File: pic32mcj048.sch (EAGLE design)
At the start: 14 parts

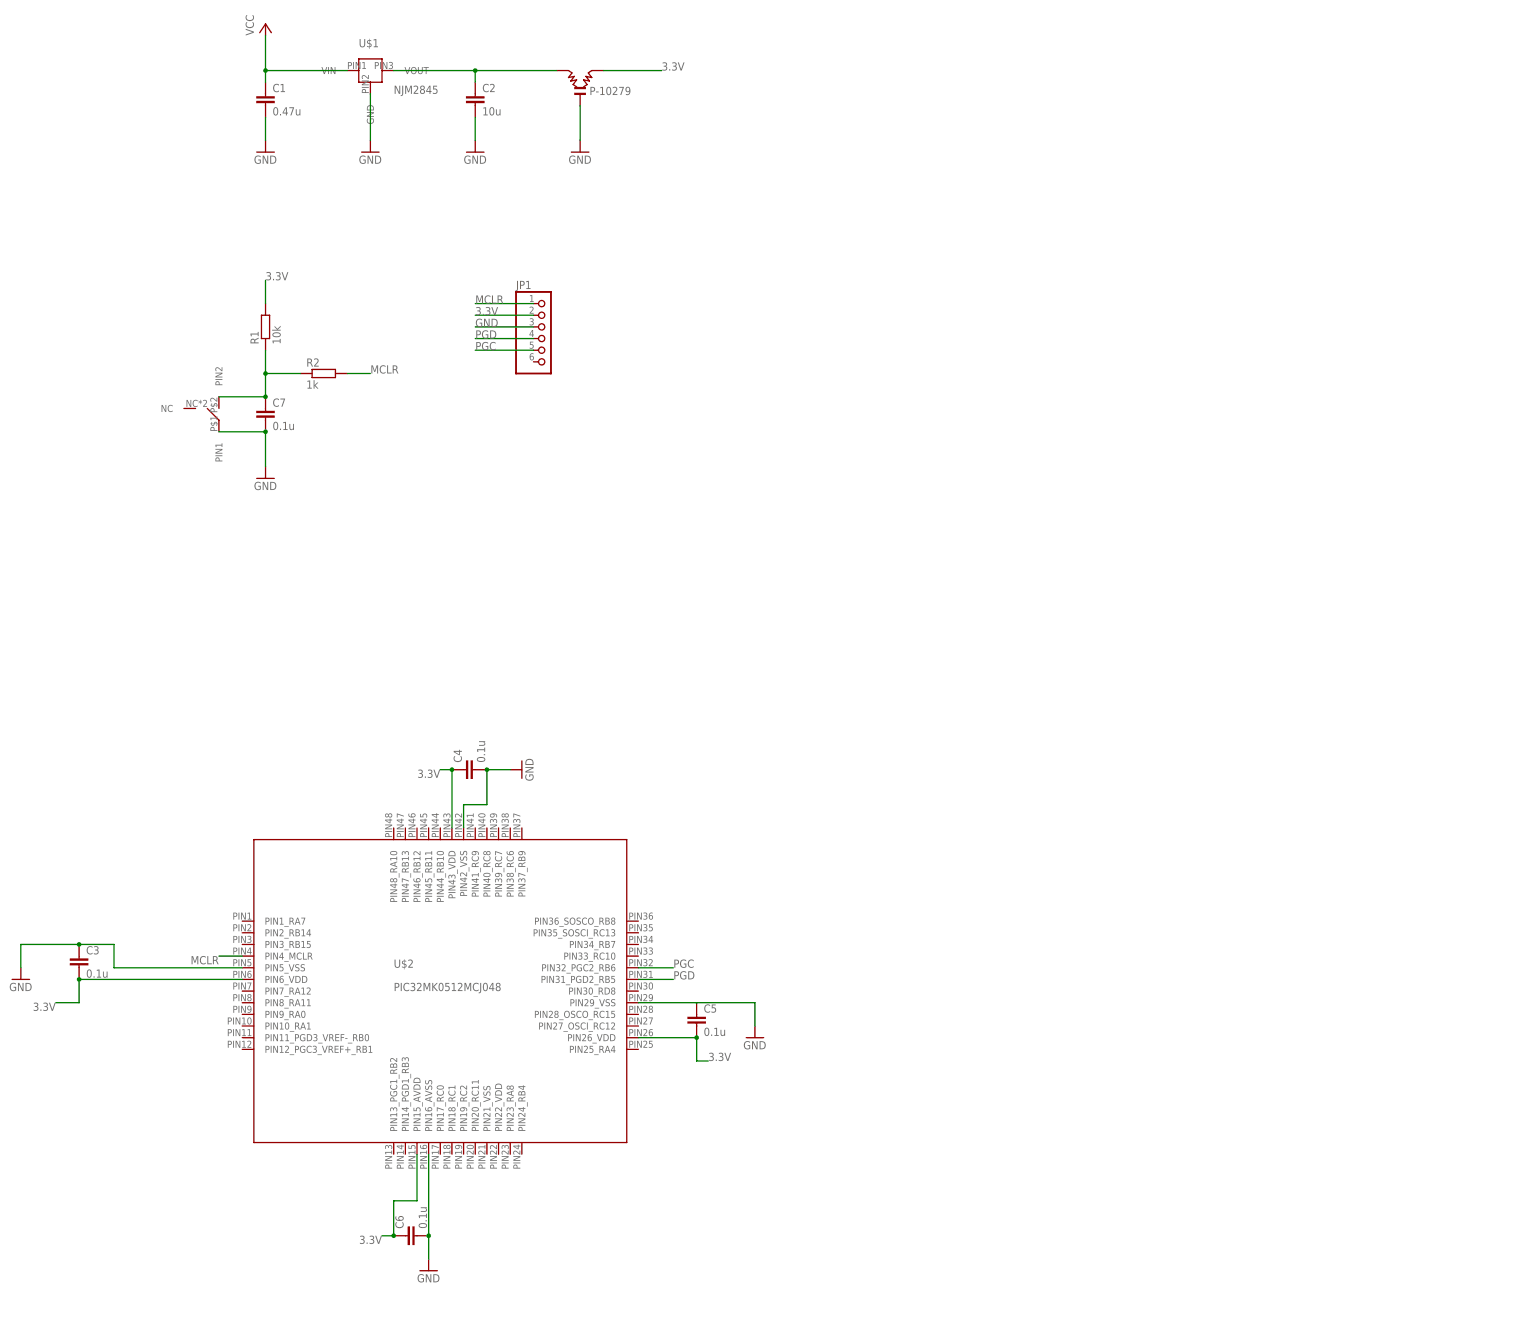
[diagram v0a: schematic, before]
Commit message: sch完成
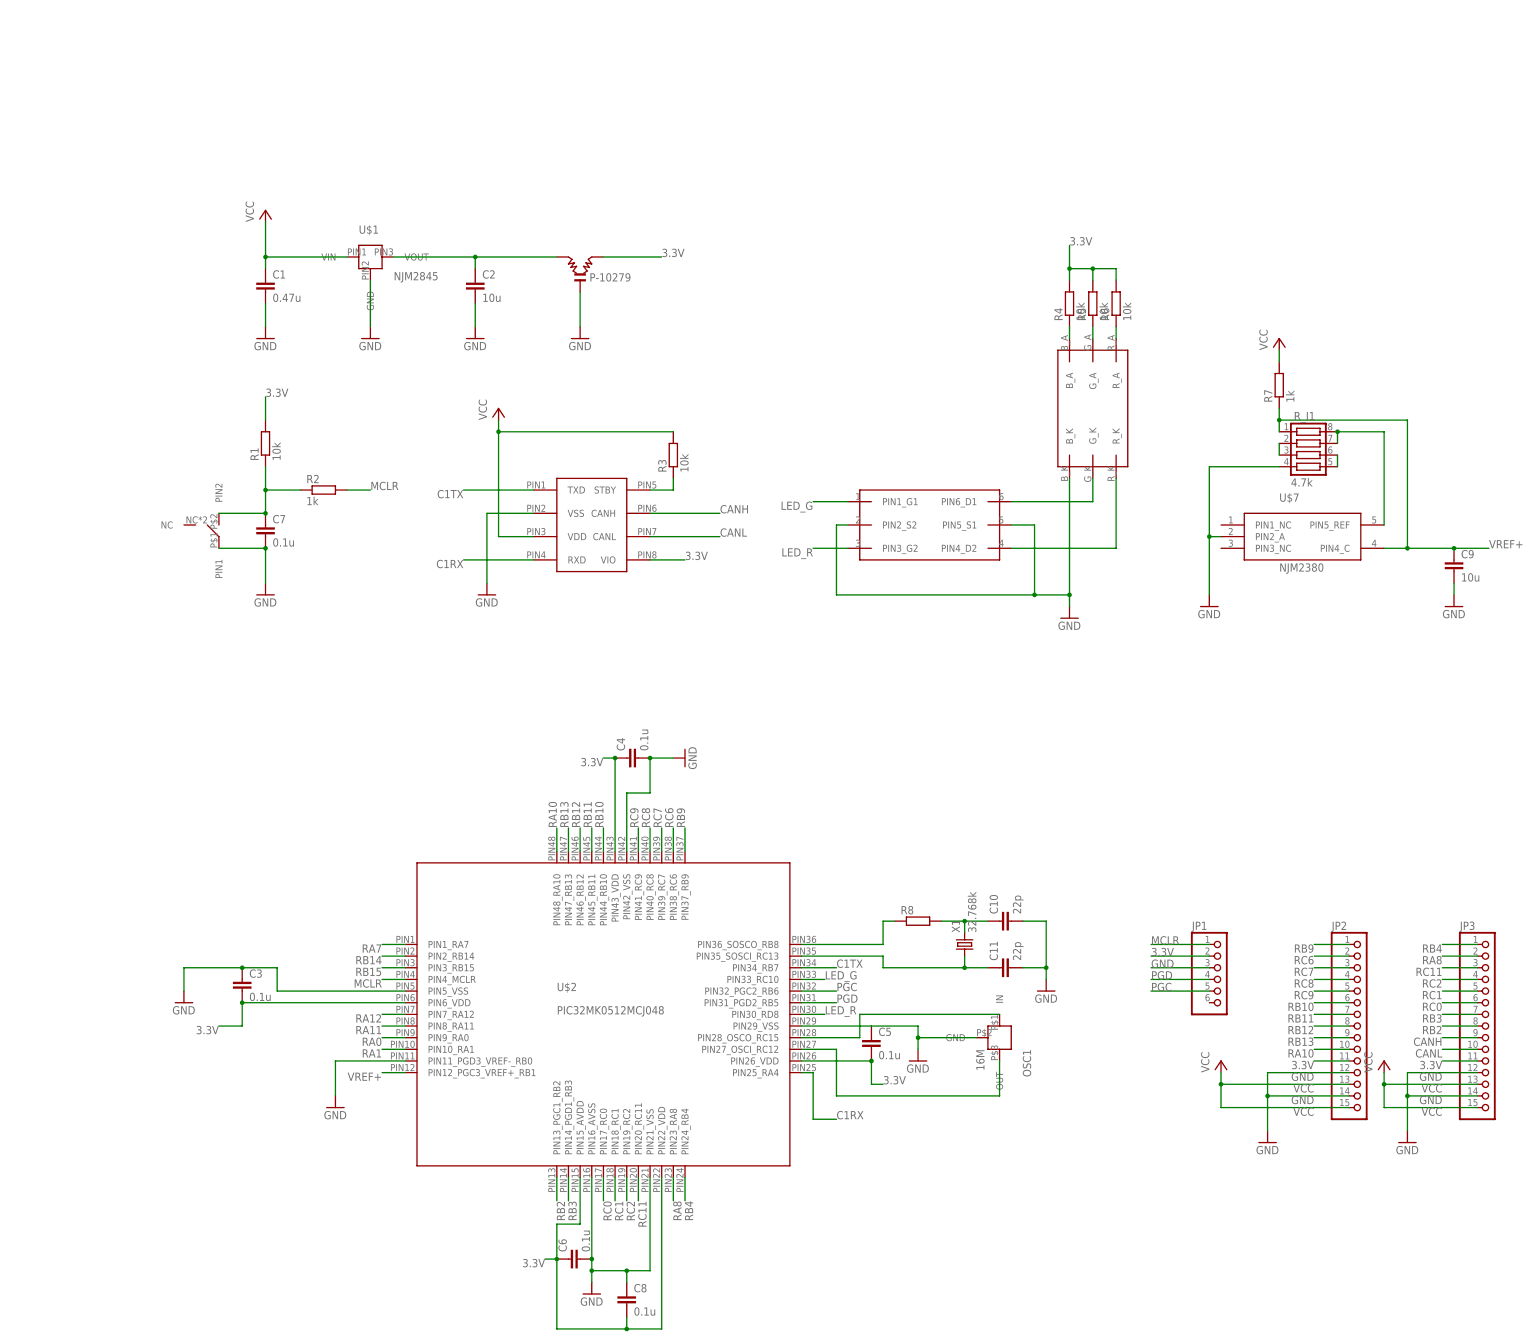
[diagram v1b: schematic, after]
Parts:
- added C10, C11: 22p, rcl:C-EUC1608
- added C8: 0.1u, rcl:C-EUC1608
- added C9: 10u, rcl:C-EUC1608
- added IC1: (no value), user_ic:MCP2562
- added JP2, JP3: (no value), pinhead:PINHD-1X15
- added OSC1: 16M, user_osc:CSTN#
- added R3, R4, R5, R6: 10k, user_rcl:R_REG
- added R7: 1k, user_rcl:R_REG
- added R8: (no value), user_rcl:R_REG
- added R_I1: 4.7k, user_rcl:R_SHUGOU2
- added U$5: RGB_LED, user_leds:RGB_LED
- added U$6: FDC6305, user_tr_fet_igbt:FDC6305
- added U$7: NJM2380, user_ic:NJM2380
- added X1: 32.768k, user_osc:FC255
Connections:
- new net C1RX: IC1.RXD, U$2.PIN25_RA4
- new net C1TX: IC1.TXD, U$2.PIN34_RB7
- new net CANH: IC1.CANH, JP3.9
- new net CANL: IC1.CANL, JP3.10
- new net LED_G: U$2.PIN33_RC10, U$6.PIN1_G1
- new net LED_R: U$2.PIN30_RD8, U$6.PIN3_G2
- new net N$11: R8.1, U$2.PIN36_SOSCO_RB8
- new net N$13: R4.1, U$5.B_A
- new net N$14: R5.1, U$5.G_A
- new net N$15: R6.1, U$5.R_A
- new net N$21: R_I1.7, R_I1.8, U$7.PIN5_REF
- new net N$3: OSC1.IN, U$2.PIN28_OSCO_RC15
- new net N$4: OSC1.OUT, U$2.PIN27_OSCI_RC12
- new net N$45: R_I1.2, R_I1.3
- new net N$46: R_I1.5, R_I1.6
- new net N$5: IC1.STBY, R3.1
- new net N$6: C10.1, R8.2, X1.2
- new net N$7: C11.1, U$2.PIN35_SOSCI_RC13, X1.1
- new net N$8: U$5.G_K, U$6.PIN6_D1
- new net N$9: U$5.R_K, U$6.PIN4_D2
- new net RA0: U$2.PIN9_RA0
- new net RA1: U$2.PIN10_RA1
- new net RA10: JP2.10, U$2.PIN48_RA10
- new net RA11: U$2.PIN8_RA11
- new net RA12: U$2.PIN7_RA12
- new net RA7: U$2.PIN1_RA7
- new net RA8: JP3.2, U$2.PIN23_RA8
- new net RB10: JP2.6, U$2.PIN44_RB10
- new net RB11: JP2.7, U$2.PIN45_RB11
- new net RB12: JP2.8, U$2.PIN46_RB12
- new net RB13: JP2.9, U$2.PIN47_RB13
- new net RB14: U$2.PIN2_RB14
- new net RB15: U$2.PIN3_RB15
- new net RB2: JP3.8, U$2.PIN13_PGC1_RB2
- new net RB3: JP3.7, U$2.PIN14_PGD1_RB3
- new net RB4: JP3.1, U$2.PIN24_RB4
- new net RB9: JP2.1, U$2.PIN37_RB9
- new net RC0: JP3.6, U$2.PIN17_RC0
- new net RC1: JP3.5, U$2.PIN18_RC1
- new net RC11: JP3.3, U$2.PIN20_RC11
- new net RC2: JP3.4, U$2.PIN19_RC2
- new net RC6: JP2.2, U$2.PIN38_RC6
- new net RC7: JP2.3, U$2.PIN39_RC7
- new net RC8: JP2.4, U$2.PIN40_RC8
- new net RC9: JP2.5, U$2.PIN41_RC9
- new net VREF+: C9.1, R7.1, R_I1.1, U$2.PIN12_PGC3_VREF+_RB1, U$7.PIN4_C
- net 3.3V: now also C8.2, IC1.VIO, JP2.11, JP3.11, R4.2, R5.2, R6.2, U$2.PIN22_VDD
- net GND: now also C10.2, C11.2, C8.1, C9.2, IC1.VSS, JP2.12, JP2.14, JP3.12, JP3.14, OSC1.GND, R_I1.4, U$2.PIN11_PGD3_VREF-_RB0, U$2.PIN21_VSS, U$5.B_K, U$6.PIN2_S2, U$6.PIN5_S1, U$7.PIN2_A
- net VCC: now also IC1.VDD, JP2.13, JP2.15, JP3.13, JP3.15, R3.2, R7.2
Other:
- moved on the sheet: C1, C2, C3, C4, C5, C6, C7, JP1, P-10279, R1, R2, U$1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
